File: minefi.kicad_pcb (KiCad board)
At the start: 2 copper layers, 130.8 x 95.2 mm, 149 parts, among them P1 CONN_25X2, P11 CONN_1, P13 CONN_1, P16 CONN_1, P18 CONN_1, P2 CONN_25X2, P4 CONN_25, P5 CONN_3X2, P51 CONN_1, P52 CONN_1, Q1001 MOS_PRO, Q401 OVP_DRIVER, Q402 OVP_DRIVER, Q403 OVP_DRIVER, Q404 OVP_DRIVER, U1001 LM2596, U101 MAX9926/9927, U201 MCP6004, U202 MCP6004

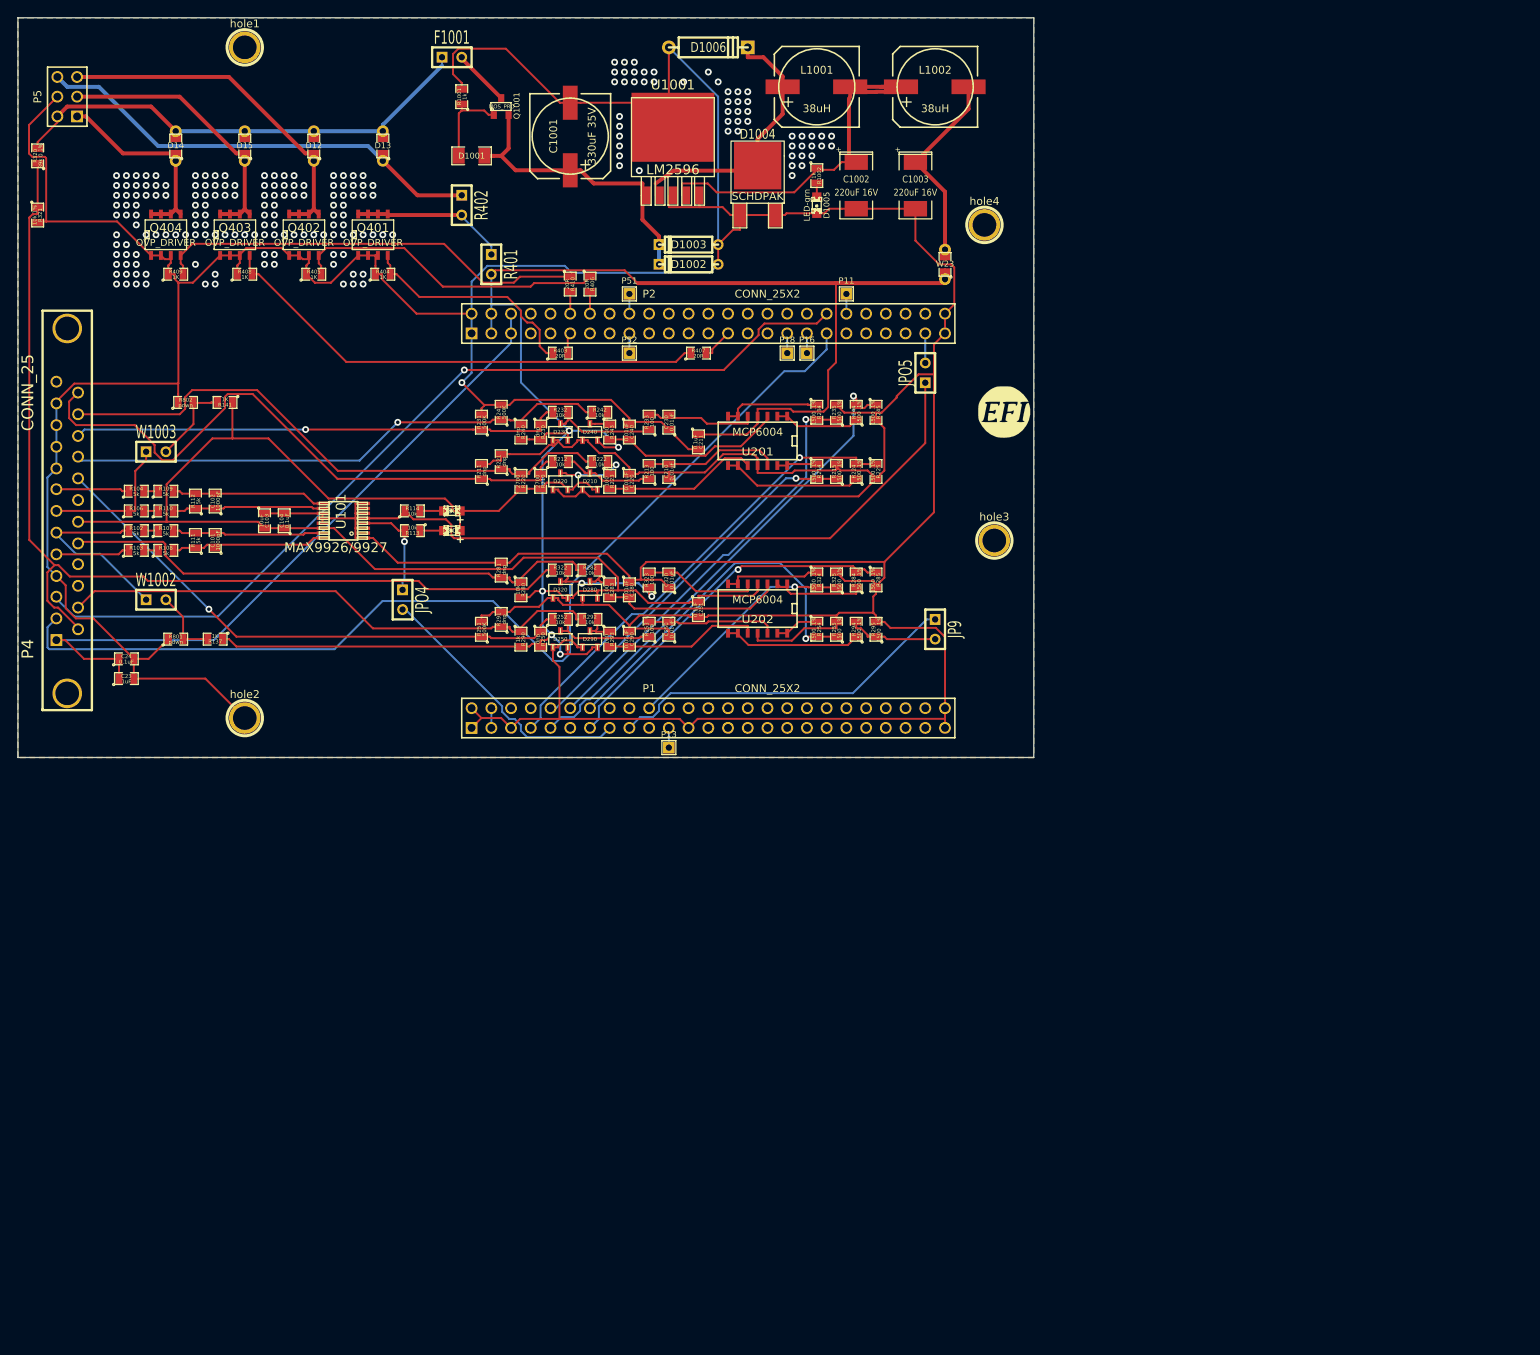
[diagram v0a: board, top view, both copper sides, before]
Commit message: wider wires
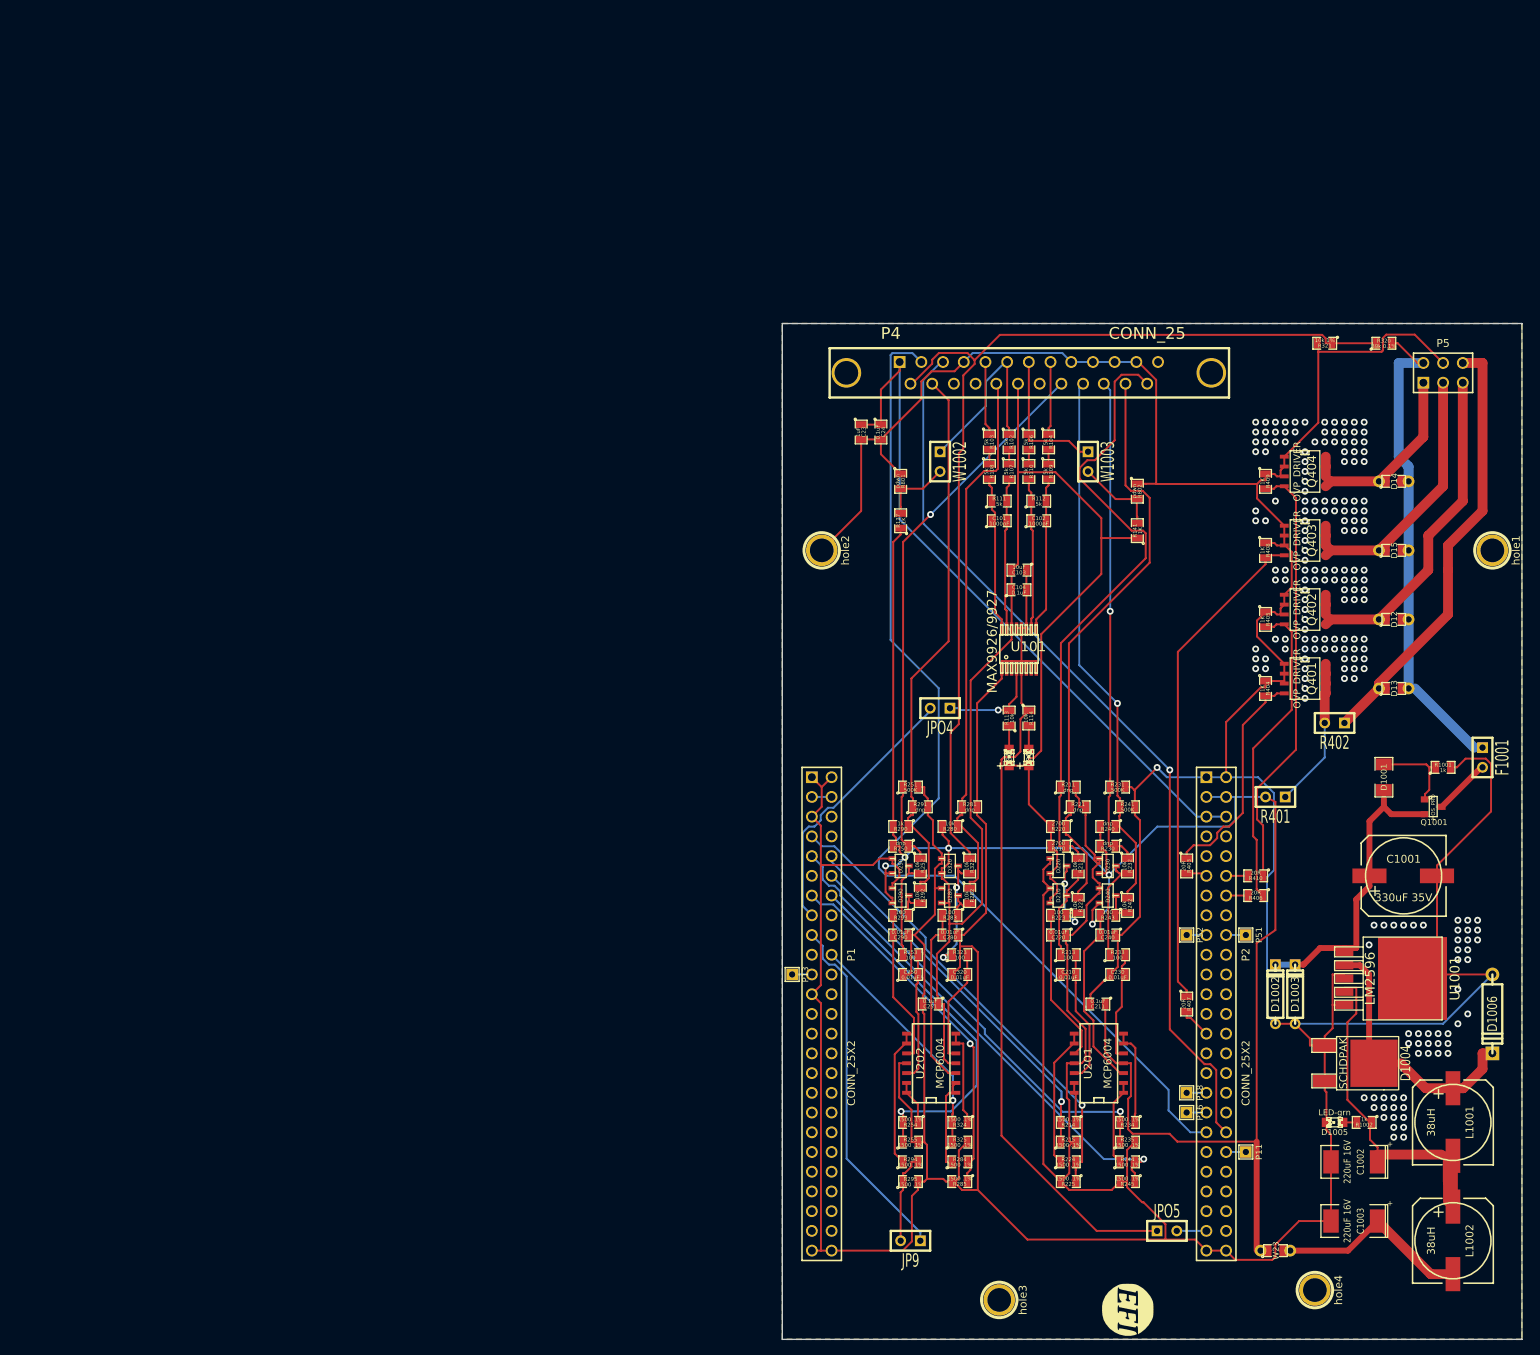
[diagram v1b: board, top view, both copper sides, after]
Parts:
- moved P5 180.7 mm to (183.5, 45.7), turned to 0 degrees
- moved R320 175.0 mm to (175.9, 41.9), turned to 0 degrees
- moved hole1 173.2 mm to (189.9, 68.6), turned to 270 degrees
- moved R321 166.6 mm to (168.3, 41.9), turned to 180 degrees
- moved L1002 162.9 mm to (184.8, 157.5), turned to 270 degrees
- moved D14 162.7 mm to (177.2, 59.7), turned to 0 degrees
- moved F1001 160.4 mm to (188.6, 95.2), turned to 270 degrees
- moved D1006 160.3 mm to (189.9, 128.3), turned to 270 degrees
- moved D15 156.9 mm to (177.2, 68.6), turned to 0 degrees
- moved L1001 156.5 mm to (184.8, 142.2), turned to 270 degrees
- moved R1001 153.1 mm to (183.5, 96.5), turned to 0 degrees
- moved D12 151.8 mm to (177.2, 77.5), turned to 0 degrees
- moved Q1001 150.1 mm to (182.2, 101.6), turned to 270 degrees
- moved Q404 149.8 mm to (165.7, 58.4), turned to 270 degrees
- moved D13 147.7 mm to (177.2, 86.4), turned to 0 degrees
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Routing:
- net /PWR_buck_12V_switcher/FB: track 51.9 -> 49.4 mm
- net /adc_amp_divider/12V_bat: track 65.4 -> 67.6 mm
- net /inj_12ch/INJ-01_2: track 59.3 -> 57.2 mm
- net /inj_12ch/INJ-02: track 46.1 -> 47.5 mm
- net /adc_amp_divider/5V: track 413.6 -> 414.7 mm
- net /inj_12ch/INJ-01: track 20.0 -> 19.5 mm
- net (no net): vias 196 -> 190
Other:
- board size 130.8 x 95.2 mm -> 95.3 x 130.8 mm
- net class power: trace_width 0.508 -> 0.762
